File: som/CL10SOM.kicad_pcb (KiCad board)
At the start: 4 copper layers, 34.9 x 31.1 mm, 53 parts, among them IC1 10CL025YU256C8G, J1 Conn_01x02_Pin, U1 MT46H32M16LFBF-5 IT:C, U2 MX25L12833FM2, U6 AT93C46DN-SH-T, U7 SG3225CAN 50.0000M-TJGA6, X1 DF40C-120DS-0.4V51

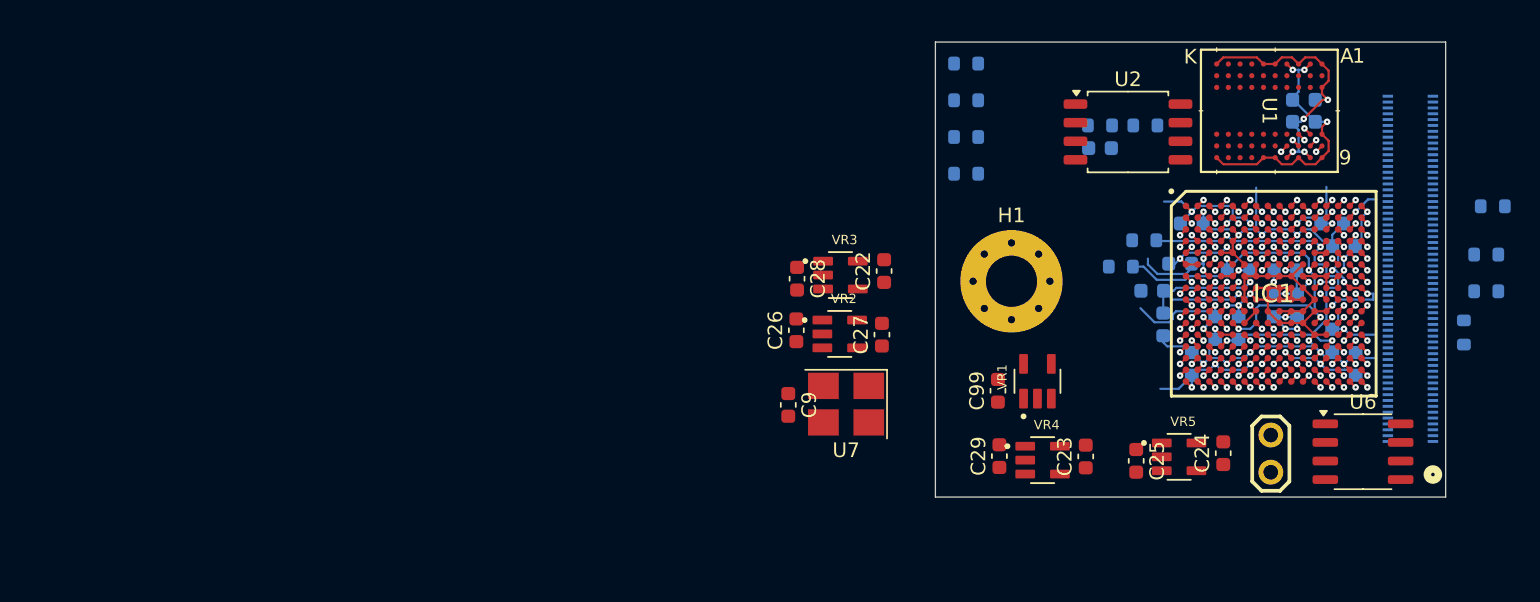
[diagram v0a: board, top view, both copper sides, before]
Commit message: Work in progress
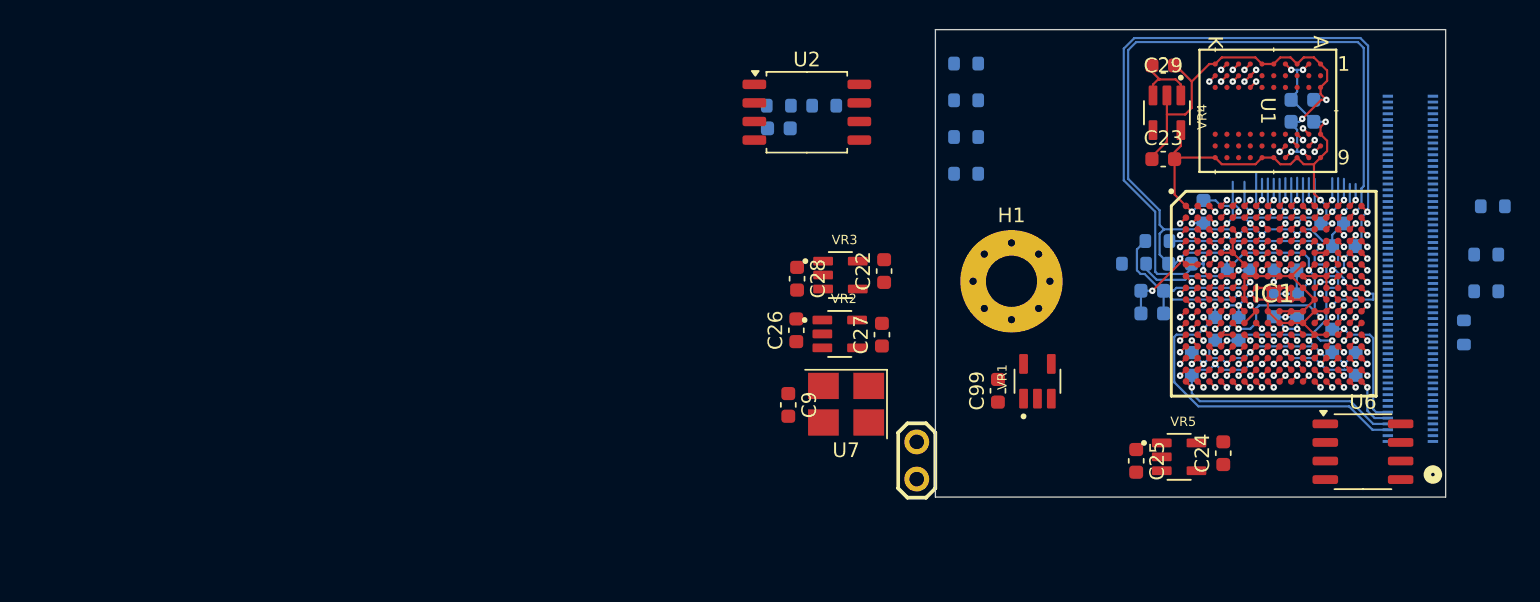
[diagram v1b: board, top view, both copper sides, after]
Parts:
- moved C29 29.0 mm to (160.3, 41.9), turned to 180 degrees
- moved VR4 25.2 mm to (160.6, 45.1), turned to -90 degrees
- moved J1 24.2 mm to (143.5, 70.1)
- moved C16 22.0 mm to (134.1, 46.1)
- moved R49 22.0 mm to (134.1, 44.6)
- moved R60 22.0 mm to (137.2, 44.6)
- moved U2 22.0 mm to (136.0, 45.0)
- moved C23 21.0 mm to (160.3, 48.2), turned to 0 degrees
- moved C12 1.13 mm to (163.1, 51.9), turned to -90 degrees
- moved C13 1.06 mm to (159.6, 58.8), turned to 180 degrees
- moved R44 0.92 mm to (158.3, 55.4)
- moved R68 0.90 mm to (159.9, 53.9)
- moved C40 0.10 mm to (169.9, 45.7)
- moved C42 0.10 mm to (169.9, 44.2)
- moved U1 0.10 mm to (167.5, 45.0)
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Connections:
- C7 pad 1: +3.3V -> +3V3
- IC1 pad A12: /DDR_A11 -> /DDR_A1
- IC1 pad A13: /DDR_A6 -> /DDR_A3
- IC1 pad A15: /DDR_A4 -> /DDR_BA1
- IC1 pad A16: +3.3V -> +3V3
- IC1 pad A2: /DDR_BA1 -> /DDR_A4
- IC1 pad A4: /DDR_A1 -> /DDR_A6
- IC1 pad A5: /DDR_DQ5 -> /DDR_A9
- IC1 pad A6: /DDR_A3 -> /DDR_CKE
- IC1 pad B13: /DDR_A9 -> /DDR_DQ5
- IC1 pad B14: /DDR_A7 -> /~{DDR_RAS}
- IC1 pad B3: /~{DDR_RAS} -> /DDR_A7
- IC1 pad B4: /DDR_CKE -> /DDR_A11
- IC1 pad E14: +3.3V -> +3V3
- IC1 pad G14: +3.3V -> +3V3
- X1 pad 10: /X1_10 -> VCCB4
- X1 pad 12: /X1_12 -> VCCB5
- X1 pad 13: /X1_13 -> unconnected-(X1-Pad13)
- X1 pad 14: /X1_14 -> unconnected-(X1-Pad14)
- X1 pad 15: /X1_15 -> unconnected-(X1-Pad15)
- X1 pad 16: /X1_16 -> unconnected-(X1-Pad16)
- X1 pad 17: /X1_17 -> unconnected-(X1-Pad17)
- X1 pad 18: /X1_18 -> unconnected-(X1-Pad18)
- X1 pad 19: /X1_19 -> unconnected-(X1-Pad19)
- X1 pad 2: /X1_2 -> GND
- X1 pad 20: /X1_20 -> unconnected-(X1-Pad20)
- X1 pad 21: /X1_21 -> unconnected-(X1-Pad21)
- X1 pad 22: /X1_22 -> unconnected-(X1-Pad22)
- X1 pad 23: /X1_23 -> unconnected-(X1-Pad23)
- X1 pad 24: /X1_24 -> unconnected-(X1-Pad24)
- X1 pad 25: /X1_25 -> unconnected-(X1-Pad25)
- X1 pad 26: /X1_26 -> unconnected-(X1-Pad26)
- X1 pad 27: /X1_27 -> unconnected-(X1-Pad27)
- X1 pad 28: /X1_28 -> unconnected-(X1-Pad28)
- X1 pad 29: /X1_29 -> unconnected-(X1-Pad29)
- X1 pad 3: /TCK -> GND
- X1 pad 30: /X1_30 -> unconnected-(X1-Pad30)
- X1 pad 31: /X1_31 -> unconnected-(X1-Pad31)
- X1 pad 32: /X1_32 -> unconnected-(X1-Pad32)
- X1 pad 33: /X1_33 -> unconnected-(X1-Pad33)
- X1 pad 34: /X1_34 -> unconnected-(X1-Pad34)
- X1 pad 35: /X1_35 -> unconnected-(X1-Pad35)
- X1 pad 36: /X1_36 -> unconnected-(X1-Pad36)
- X1 pad 37: /X1_37 -> unconnected-(X1-Pad37)
- X1 pad 38: /X1_38 -> unconnected-(X1-Pad38)
- X1 pad 39: /X1_39 -> unconnected-(X1-Pad39)
- X1 pad 4: /X1_4 -> GND
- X1 pad 40: /X1_40 -> unconnected-(X1-Pad40)
- X1 pad 5: /TDO -> unconnected-(X1-Pad5)
- X1 pad 6: /X1_6 -> VCCB2
- X1 pad 7: /TMS -> unconnected-(X1-Pad7)
- X1 pad 8: /X1_8 -> VCCB3
- X1 pad 9: /TDI -> unconnected-(X1-Pad9)
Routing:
- net GND: track 123.4 -> 180.4 mm, vias 31 -> 32
- net +3V3: track 6.31 -> 58.3 mm, vias 2 -> 7
- net /DDR_CLK: track 0.57 -> 24.2 mm, vias 2 -> 4
- net /~{DDR_CLK}: track 0.57 -> 18.0 mm, vias 1 -> 2
- net VCCB2: track 9.16 -> 24.3 mm
- net VCCB3: track 9.72 -> 21.9 mm
- net +1V8: track 35.6 -> 46.9 mm, vias 8 -> 9
- net /DDR_A7: track 0.57 -> 11.7 mm, vias 2 -> 4
- net /DDR_A11: track 0.57 -> 10.5 mm, vias 1 -> 3
- net /DDR_A4: track 0.57 -> 10.2 mm, vias 2 -> 4
- net /DDR_CKE: track 0.57 -> 10.2 mm, vias 1 -> 2
- net /DDR_A9: track 0.57 -> 10.2 mm, vias 2 -> 4
- net /DDR_A6: track 0.57 -> 10.2 mm, vias 2 -> 4
- net +3.3V: track 8.36 -> 0.00 mm, vias 5 -> 0
- net /~{DDR_WE}: track 0.57 -> 8.83 mm
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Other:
- board size 34.9 x 31.1 mm -> 34.9 x 31.9 mm

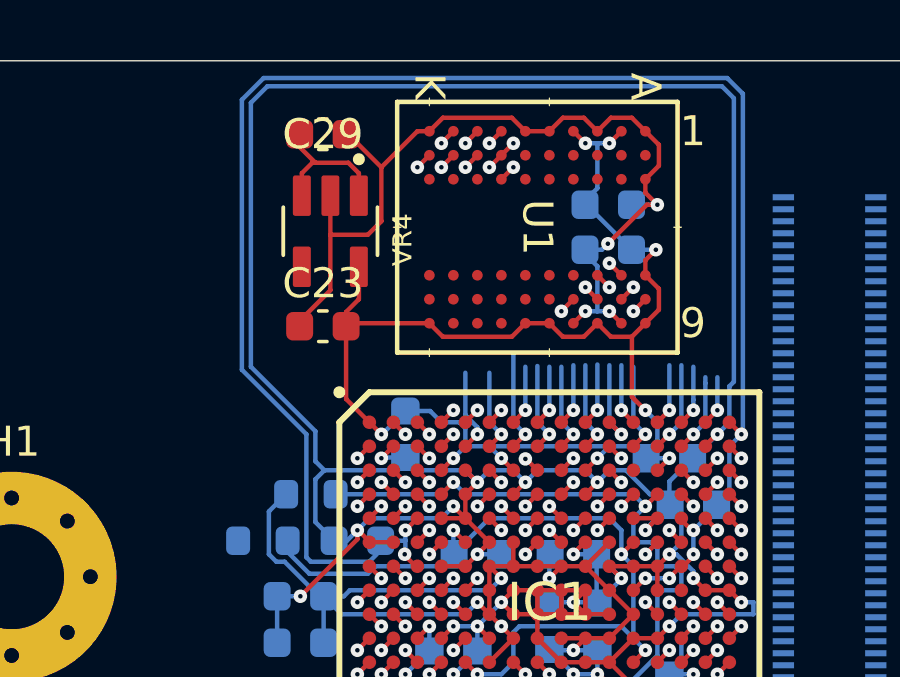
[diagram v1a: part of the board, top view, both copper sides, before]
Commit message: Work in progress
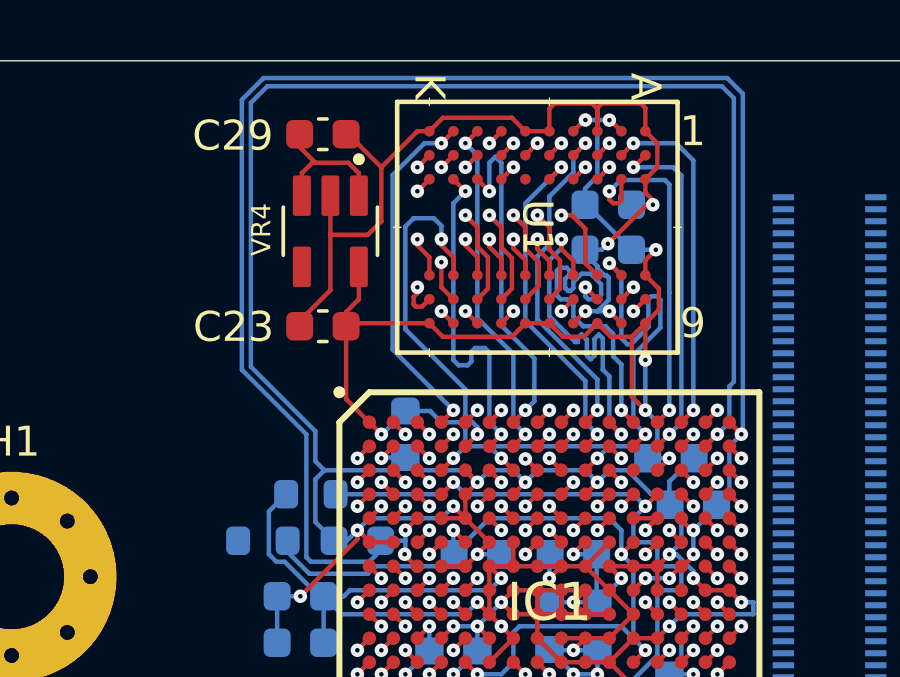
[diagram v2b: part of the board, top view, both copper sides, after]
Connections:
- IC1 pad A10: /~{DDR_CAS} -> /DDR_DQ9
- IC1 pad A11: /DDR_A8 -> /DDR_DQ5
- IC1 pad A12: /DDR_A1 -> /DDR_DQ4
- IC1 pad A13: /DDR_A3 -> /DDR_DQ14
- IC1 pad A14: /DDR_A10 -> /DDR_DQ13
- IC1 pad A15: /DDR_BA1 -> /DDR_DQ12
- IC1 pad A3: /DDR_A12 -> /DDR_A5
- IC1 pad A5: /DDR_A9 -> /DDR_A1
- IC1 pad A6: /DDR_CKE -> /~{DDR_CAS}
- IC1 pad A7: /DDR_DQ7 -> /DDR_A12
- IC1 pad B10: /DDR_DQ11 -> /DDR_DQ8
- IC1 pad B11: /DDR_DQ15 -> /DDR_DQ3
- IC1 pad B12: /DDR_A2 -> /DDR_DQ1
- IC1 pad B13: /DDR_DQ5 -> /DDR_DQ15
- IC1 pad B14: /~{DDR_RAS} -> /DDR_DQ11
- IC1 pad B5: /DDR_DQ3 -> /DDR_A10
- IC1 pad B6: /DDR_DQ2 -> /DDR_A8
- IC1 pad B7: /DDR_A5 -> /DDR_A9
- IC1 pad C11: /DDR_DQ9 -> /DDR_DQ10
- IC1 pad C14: /DDR_DM1 -> /DDR_DQ0
- IC1 pad C6: /DDR_DQ1 -> /DDR_BA0
- IC1 pad C8: /DDR_A13 -> /DDR_CKE
- IC1 pad C9: /DDR_DQ12 -> /DDR_DQS1
- IC1 pad D11: /DDR_BA0 -> /DDR_DQS0
- IC1 pad D12: /DDR_A0 -> /DDR_DM1
- IC1 pad D14: /DDR_DM0 -> /DDR_DQ2
- IC1 pad D6: /DDR_DQ4 -> /DDR_A2
- IC1 pad D8: /DDR_DQ6 -> /~{DDR_RAS}
- IC1 pad D9: /DDR_DQ8 -> /DDR_DM0
- IC1 pad E10: /DDR_DQ14 -> /DDR_DQ7
- IC1 pad E11: /~{DDR_CS} -> /DDR_DQ6
- IC1 pad E6: /~{DDR_WE} -> /DDR_A3
- IC1 pad E7: /DDR_DQS0 -> /~{DDR_CS}
- IC1 pad E8: /DDR_DQS1 -> /DDR_A0
- IC1 pad E9: /DDR_DQ13 -> /~{DDR_WE}
- IC1 pad F8: /DDR_DQ0 -> /DDR_A13
- IC1 pad F9: /DDR_DQ10 -> /DDR_BA1
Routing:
- net /DDR_DQ7: track 2.02 -> 14.4 mm
- net /DDR_A1: track 2.07 -> 14.3 mm, vias 0 -> 2
- net /DDR_A2: track 2.98 -> 14.2 mm
- net /DDR_A5: track 3.41 -> 14.3 mm, vias 1 -> 2
- net /DDR_DQ2: track 3.35 -> 14.2 mm, vias 3 -> 2
- net /DDR_DQ12: track 4.41 -> 14.6 mm
- net /DDR_A3: track 2.07 -> 12.2 mm, vias 0 -> 2
- net /DDR_BA1: track 1.67 -> 11.7 mm, vias 1 -> 2
- net /~{DDR_CAS}: track 2.09 -> 12.0 mm
- net /DDR_A13: track 4.44 -> 14.3 mm
- net /DDR_A10: track 2.02 -> 11.7 mm
- net /DDR_DQ11: track 3.03 -> 12.3 mm
- net /DDR_DM1: track 5.74 -> 14.7 mm, vias 1 -> 2
- net /DDR_A0: track 5.56 -> 14.5 mm
- net /DDR_DQ3: track 3.35 -> 12.2 mm, vias 3 -> 2
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
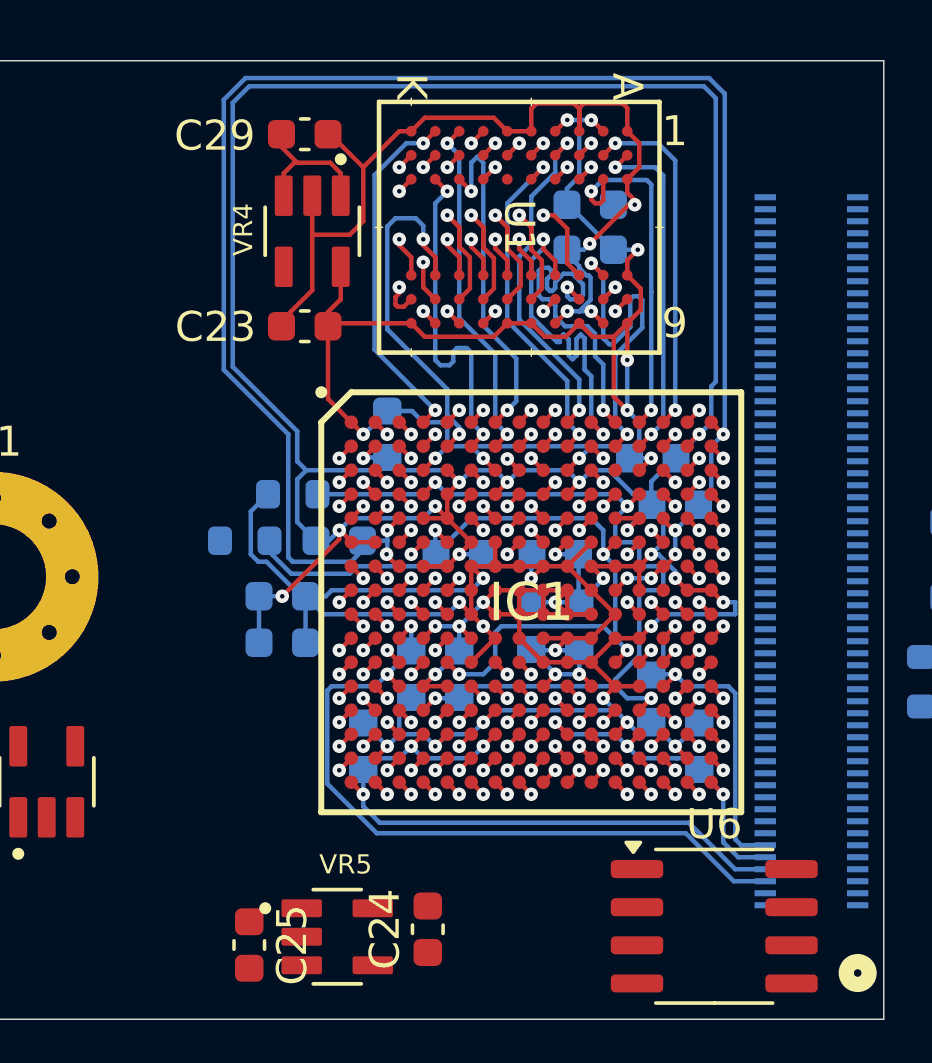
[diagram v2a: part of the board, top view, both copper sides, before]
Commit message: Work in progress
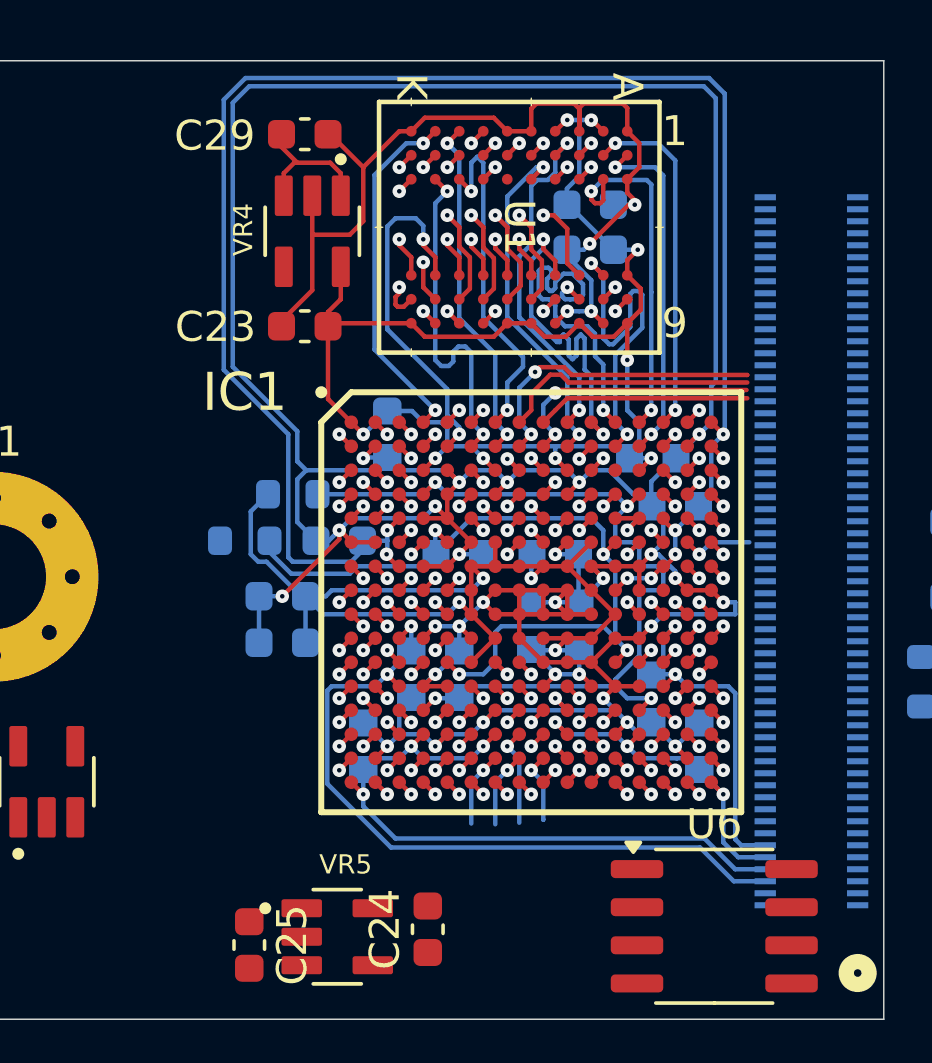
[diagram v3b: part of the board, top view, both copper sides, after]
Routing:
- net /B8-CLK11: track 0.57 -> 10.3 mm, vias 1 -> 2
- net /nCONFIG: track 0.57 -> 10.2 mm
- net /TMS: track 0.57 -> 9.17 mm
- net /TDI: track 0.57 -> 9.08 mm
- net /B1-IO2: track 0.57 -> 8.90 mm
- net /B7-CLK9: track 0.57 -> 8.69 mm, vias 1 -> 2
- net /B8-CLK10: track 0.57 -> 8.69 mm, vias 1 -> 0
- net /TCK: track 0.57 -> 8.43 mm
- net /nSTATUS: track 0.57 -> 8.26 mm
- net /B4-IO1: track 0.57 -> 7.50 mm
- net /FL_D2: track 0.57 -> 7.45 mm
- net /B4-IO6: track 0.57 -> 7.37 mm
- net /B7-CLK8: track 0.57 -> 7.13 mm, vias 1 -> 0
- net /B4-IO12: track 0.57 -> 6.84 mm
- net /B1-IO3: track 0.57 -> 6.81 mm
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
